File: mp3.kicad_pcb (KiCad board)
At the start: 2 copper layers, 58 x 79 mm, 47 parts, among them J1 AudioJack4_Ground, J2 AudioJack4_Ground, J3 Conn_01x08, J4 Micro_SD_Card_Det1, SW2 SW_Nidec_CAS-120A1, U1 XTAD5142IRGER, U2 MCP6002-xSN, U4 TP4056-42-ESOP8

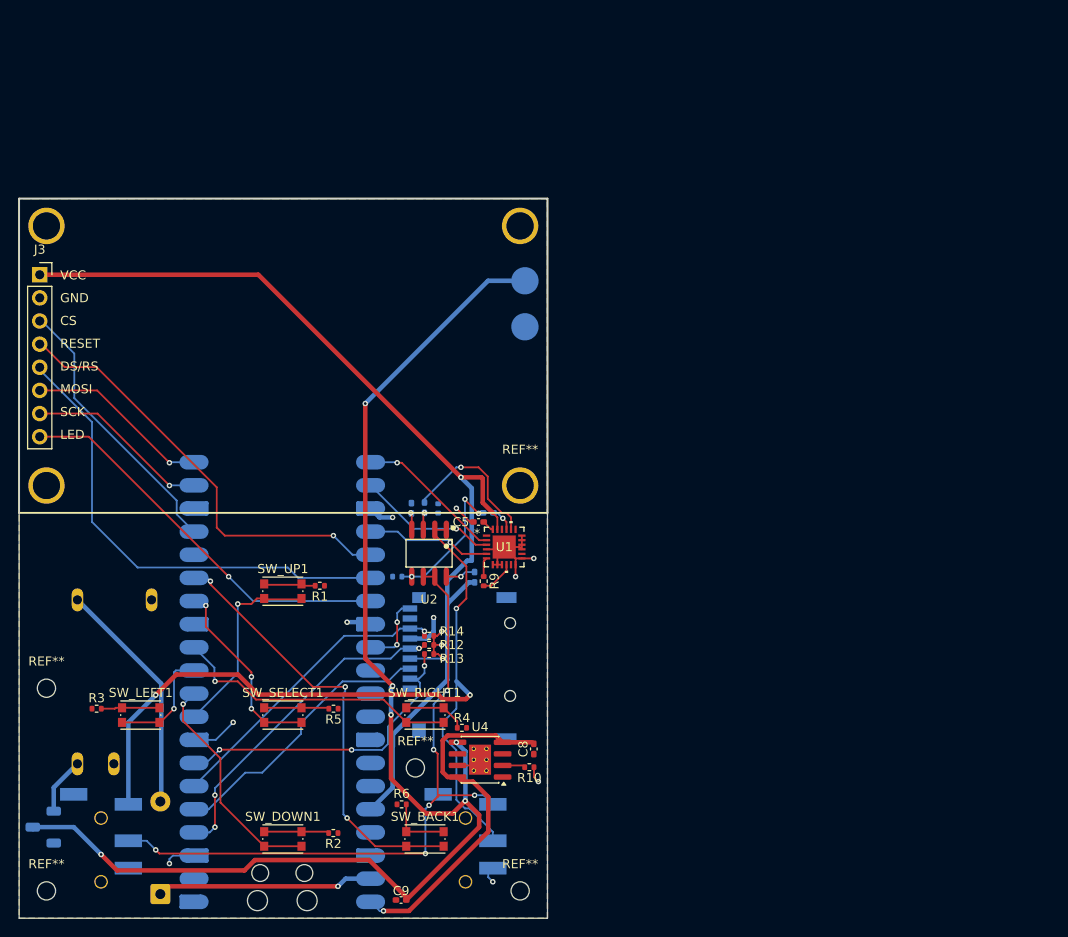
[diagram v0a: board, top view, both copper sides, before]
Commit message: Full re-routing
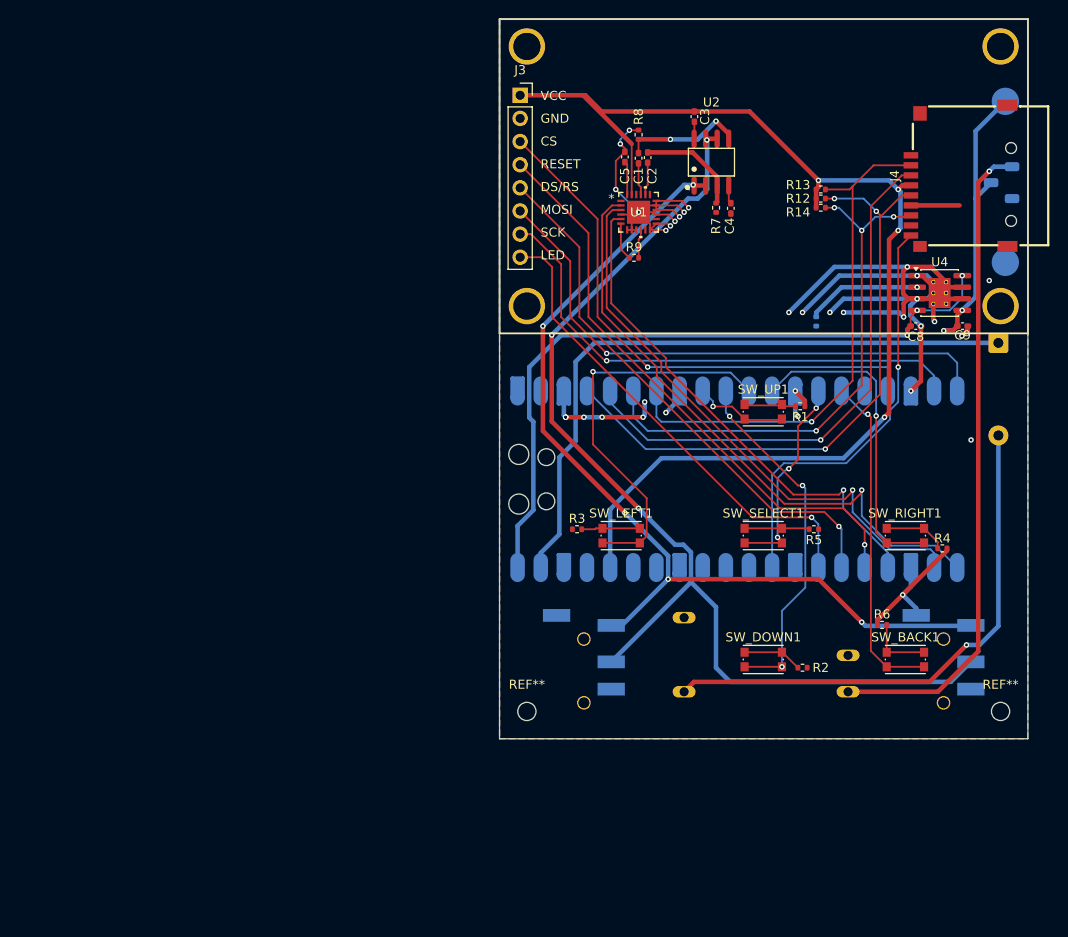
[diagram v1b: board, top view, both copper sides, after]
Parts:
- removed the REF** at (62.0, 133.5)
- removed the REF** at (73.5, 102.5)
- removed the REF** at (21.5, 124.8)
- added ?: , , F.Cu at (126.2, 82.8)
- C1, C2, C3, C4, J4, R7, R8: moved to F.Cu
- R10: moved to B.Cu
- moved SW2 126.8 mm to (126.3, 69.2)
- moved D1 110.1 mm to (126.0, 86.8), turned to -90 degrees
- moved J2 94.6 mm to (120.0, 120.8)
- moved C9 88.1 mm to (122.1, 85.0), turned to 0 degrees
- moved J4 77.1 mm to (121.7, 68.5), turned to 90 degrees
- moved U4 71.9 mm to (119.6, 81.4), turned to 0 degrees
- moved CKCS_BS-2 71.5 mm to (100.4, 121.1), turned to 180 degrees
- moved R13 66.7 mm to (106.5, 70.0), turned to 0 degrees
- moved R12 65.2 mm to (106.5, 71.0), turned to 0 degrees
- moved R14 63.7 mm to (106.5, 72.0), turned to 0 degrees
- moved C8 62.6 mm to (116.9, 85.0), turned to 180 degrees
- moved R10 58.2 mm to (106.0, 84.5), turned to 90 degrees
- moved SW_BACK1 56.3 mm to (115.8, 121.6)
- moved R1 56.3 mm to (104.2, 93.8)
- moved R5 56.3 mm to (105.8, 107.3)
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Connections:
- J1 pad 3: Net-(U2A--) -> Net-(U2B--)
- J1 pad 4: Net-(U2B--) -> Net-(U2A--)
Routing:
- net -BATT: track 45.4 -> 172.2 mm, vias 10 -> 34
- net +BATT: track 143.2 -> 32.0 mm, vias 6 -> 2
- net /CKCS_IN: track 6.28 -> 72.0 mm, vias 0 -> 1
- net /Pico_I2S_SCK: track 16.4 -> 67.4 mm
- net /Pico_I2S_FSYNC: track 15.4 -> 63.5 mm
- net Net-(A1-VSYS): track 24.7 -> 71.4 mm, vias 1 -> 0
- net Net-(U2B--): track 73.6 -> 116.8 mm, vias 6 -> 3
- net /Pico_I2S_SD: track 13.8 -> 55.7 mm
- net /SCREEN_SDI_MOSI: track 20.9 -> 61.6 mm
- net /SD_DET: track 8.11 -> 46.8 mm, vias 2 -> 1
- net /SCREEN_SCK: track 20.2 -> 57.1 mm
- net /Pico_VBUS: track 41.4 -> 77.0 mm, vias 1 -> 3
- net /Pico_VSYS: track 26.0 -> 58.4 mm, vias 0 -> 1
- net /SD_CLK: track 36.3 -> 68.1 mm
- net /BTN_LEFT: track 12.5 -> 43.6 mm
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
